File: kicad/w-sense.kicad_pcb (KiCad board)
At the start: 2 copper layers, 131 x 24 mm, 40 parts, among them Q1 MMBT3906, SW1 reset, SW2 boot, U1 ESP32-C3FH4, X1 SMD0603-4, Y1 32.768kHz

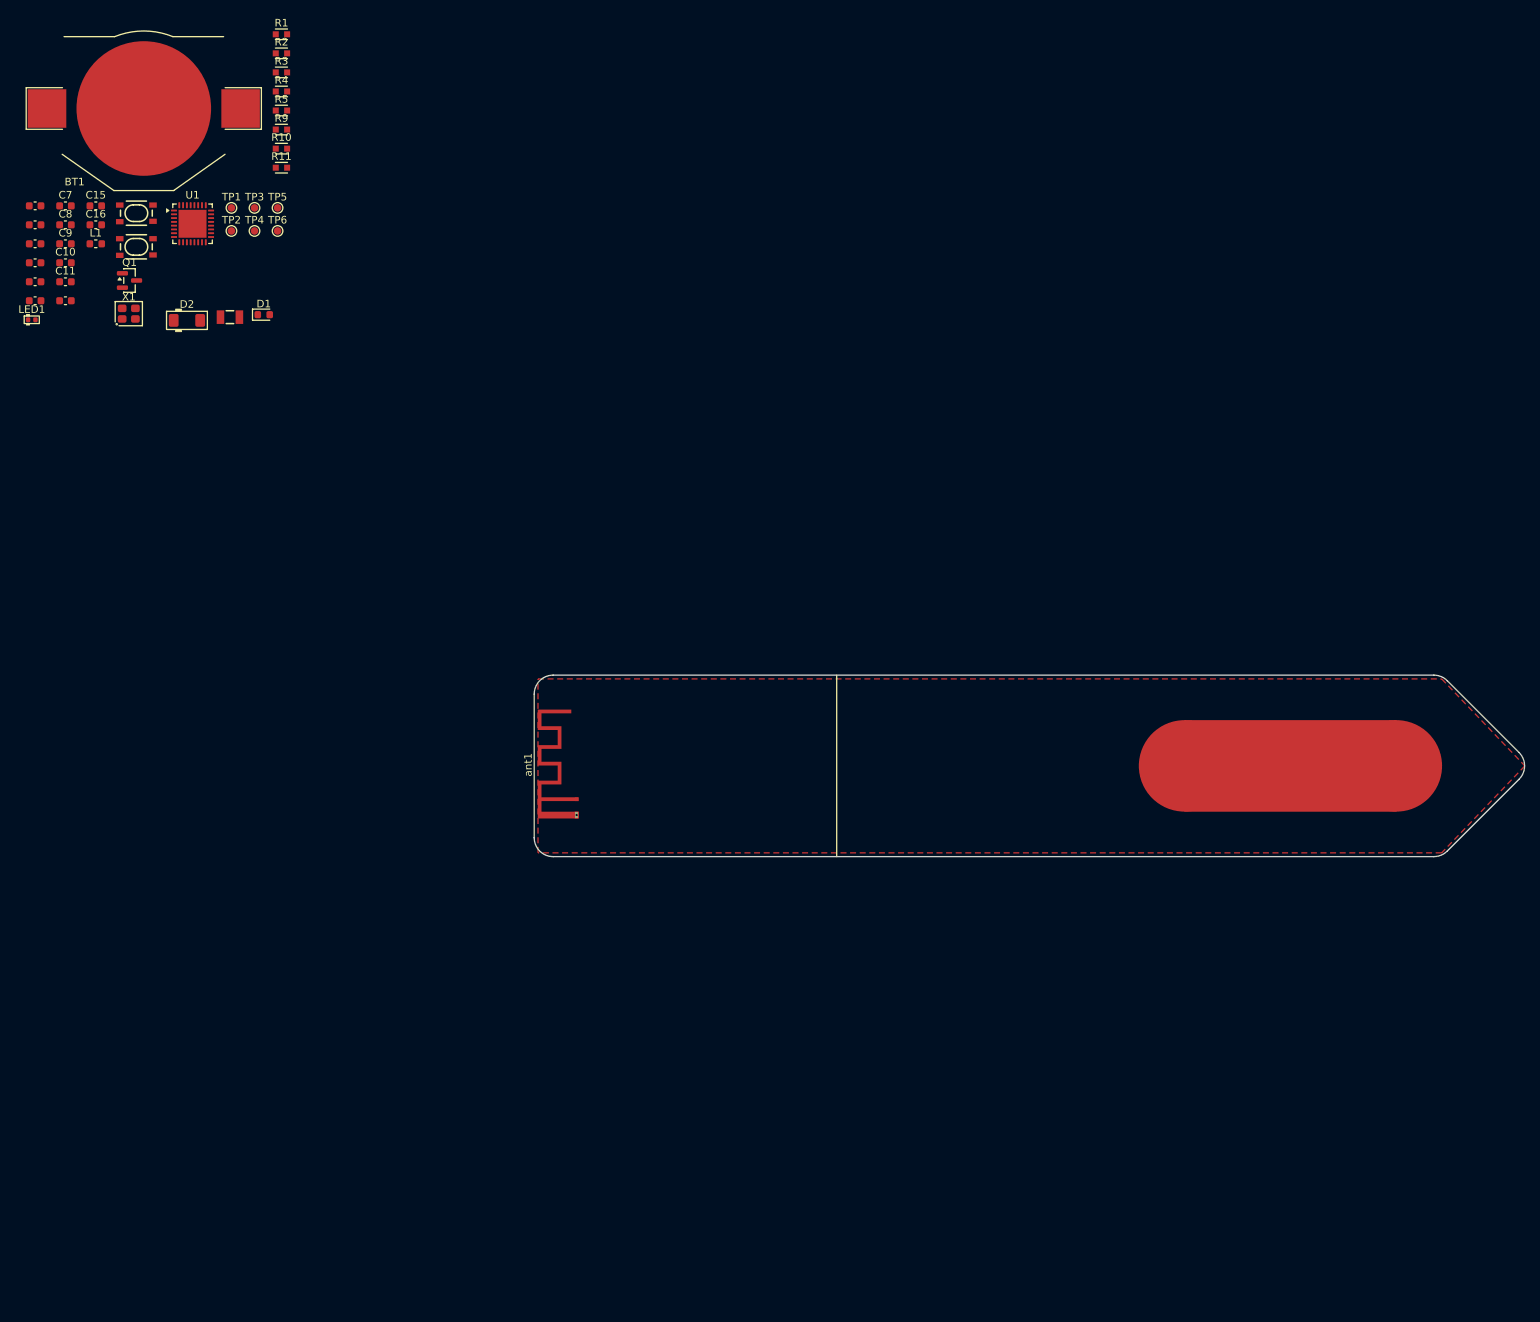
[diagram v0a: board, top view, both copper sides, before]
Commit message: finished pcb and schematic
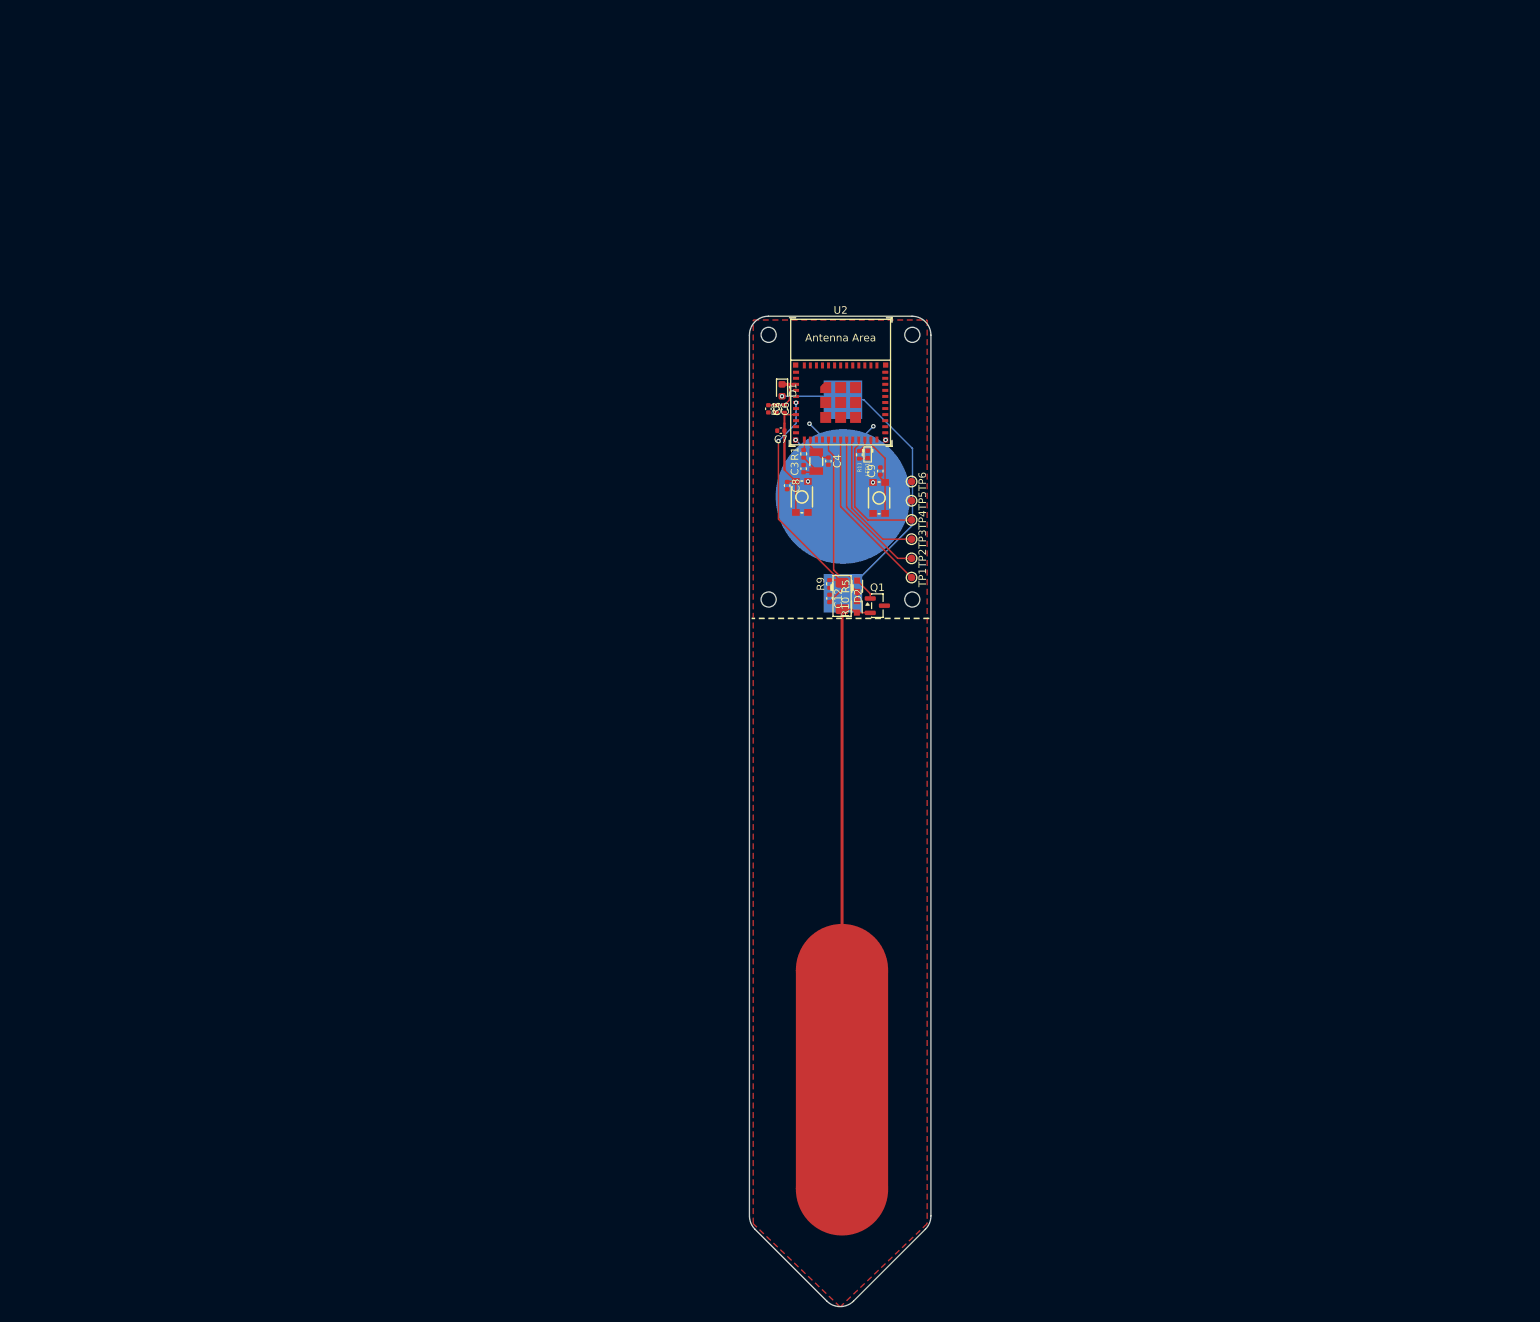
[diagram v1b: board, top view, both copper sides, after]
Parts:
- removed C1, C2: 18pF, PCM_SparkFun-Capacitor:C_0603_1608Metric
- removed C10, C11, C15, C16: 100nF, Capacitor_SMD:C_0603_1608Metric
- removed L1: 2nH, Inductor_SMD:L_0603_1608Metric
- removed R3, R4: 10K, PCM_fab:R_0603
- removed U1: ESP32-C3FH4, Package_DFN_QFN:QFN-32-1EP_5x5mm_P0.5mm_EP3.7x3.7mm
- removed X1: SMD0603-4, PCM_Crystal_AKL:Crystal_SMD_2520-4Pin_2.5x2.0mm
- removed ant1: ~, RF_Antenna:Texas_SWRA117D_2.4GHz_Right
- added U2: ESP32-C3-MINI-1, PCM_Espressif:ESP32-C3-MINI-1, F.Cu at (130.5, 61.2)
- BT1: moved to B.Cu
- C12, C3, C4: footprint PCM_SparkFun-Capacitor:C_0603_1608Metric -> Capacitor_SMD:C_0402_1005Metric
- C5, C6: value 18pF -> 0.1uF; footprint PCM_SparkFun-Capacitor:C_0603_1608Metric -> Capacitor_SMD:C_0402_1005Metric
- C7: value 100nF -> 1uF; footprint Capacitor_SMD:C_0603_1608Metric -> Capacitor_SMD:C_0402_1005Metric
- C8, C9: value 100nF -> 0.1uF; footprint Capacitor_SMD:C_0603_1608Metric -> Capacitor_SMD:C_0402_1005Metric
- R1, R11, R9: footprint PCM_fab:R_0603 -> Resistor_SMD:R_0402_1005Metric
- R2: value 0R -> 10K; footprint PCM_fab:R_0603 -> Resistor_SMD:R_0402_1005Metric
- SW1: value reset -> SMD_4.6x2.8mm_h1.9mm; footprint PCM_SparkFun-Switch:Push_SMD_4.2x3.2mm -> PCM_SparkFun-Switch:Push_SMD_4.6x2.8mm_h1.9mm
- SW2: value boot -> SMD_4.6x2.8mm_h1.9mm; footprint PCM_SparkFun-Switch:Push_SMD_4.2x3.2mm -> PCM_SparkFun-Switch:Push_SMD_4.6x2.8mm_h1.9mm
- moved LED1 112.0 mm to (134.1, 70.8), turned to -90 degrees
- moved C9 111.9 mm to (135.8, 73.0), turned to 90 degrees
- moved C12 108.4 mm to (129.0, 89.9), turned to -90 degrees
- moved C4 108.1 mm to (128.9, 71.7), turned to -90 degrees
- moved Q1 107.8 mm to (135.4, 90.8)
- moved C3 105.9 mm to (125.6, 72.7), turned to 90 degrees
- moved BT1 105.7 mm to (130.8, 76.4), turned to -90 degrees
- moved SW2 103.7 mm to (135.6, 76.6), turned to 90 degrees
- moved TP1 102.4 mm to (139.9, 87.1), turned to -90 degrees
- moved C8 101.5 mm to (123.5, 74.9), turned to -90 degrees
- moved TP2 99.8 mm to (139.9, 84.6), turned to -90 degrees
- moved C7 99.2 mm to (122.6, 67.7), turned to 180 degrees
- moved C6 99.1 mm to (122.0, 64.8), turned to -90 degrees
- moved R5 98.8 mm to (132.7, 88.2), turned to 90 degrees
- moved C5 98.4 mm to (121.0, 64.8), turned to -90 degrees
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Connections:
- C5 pad 1: /RST -> +3V0
- C6 pad 1: /BOOT -> +3V0
- C7 pad 1: +3V0 -> /EN
- C7 pad 2: Net-(C7-Pad2) -> GND
- C8 pad 1: +3V0 -> /EN
- C8 pad 2: Net-(U1-VDD_SPI) -> GND
- C9 pad 1: +3V0 -> /BOOT
- C9 pad 2: Net-(U1-VDD3P3_CPU) -> GND
- R2 pad 1: Net-(C2-Pad2) -> /EN
- R2 pad 2: /P -> +3V0
- SW1 pad 2: /RST -> /EN
- TP6 pad 1: +3V0 -> +3V3
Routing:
- net GND: track 0.00 -> 52.5 mm, vias 0 -> 6
- net /PROBE: track 0.00 -> 51.8 mm
- net Net-(BT1-+): track 0.00 -> 43.2 mm, vias 0 -> 1
- net /AOUT: track 0.00 -> 33.3 mm, vias 0 -> 2
- net /EN: track 0.00 -> 30.4 mm
- net /pwm: track 0.00 -> 23.7 mm
- net /MTMS: track 0.00 -> 22.1 mm
- net /MTDI: track 0.00 -> 20.3 mm
- net /MTCK: track 0.00 -> 18.7 mm
- net /MTDO: track 0.00 -> 17.4 mm
- net /BOOT: track 0.00 -> 11.8 mm
- net +3V0: track 0.00 -> 6.99 mm
- net Net-(C3-Pad1): track 0.00 -> 4.19 mm
- net /32K_N: track 0.00 -> 3.89 mm
- net Net-(Q1-B): track 0.00 -> 3.08 mm
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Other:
- board size 131 x 24 mm -> 24 x 131 mm
